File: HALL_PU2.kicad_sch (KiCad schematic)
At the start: 21 parts, among them Q15 AO3400A, Q16 AO3401A, Q17 AO3401A, Q2 AO3400A, Q4 AO3401A, Q5 AO3401A

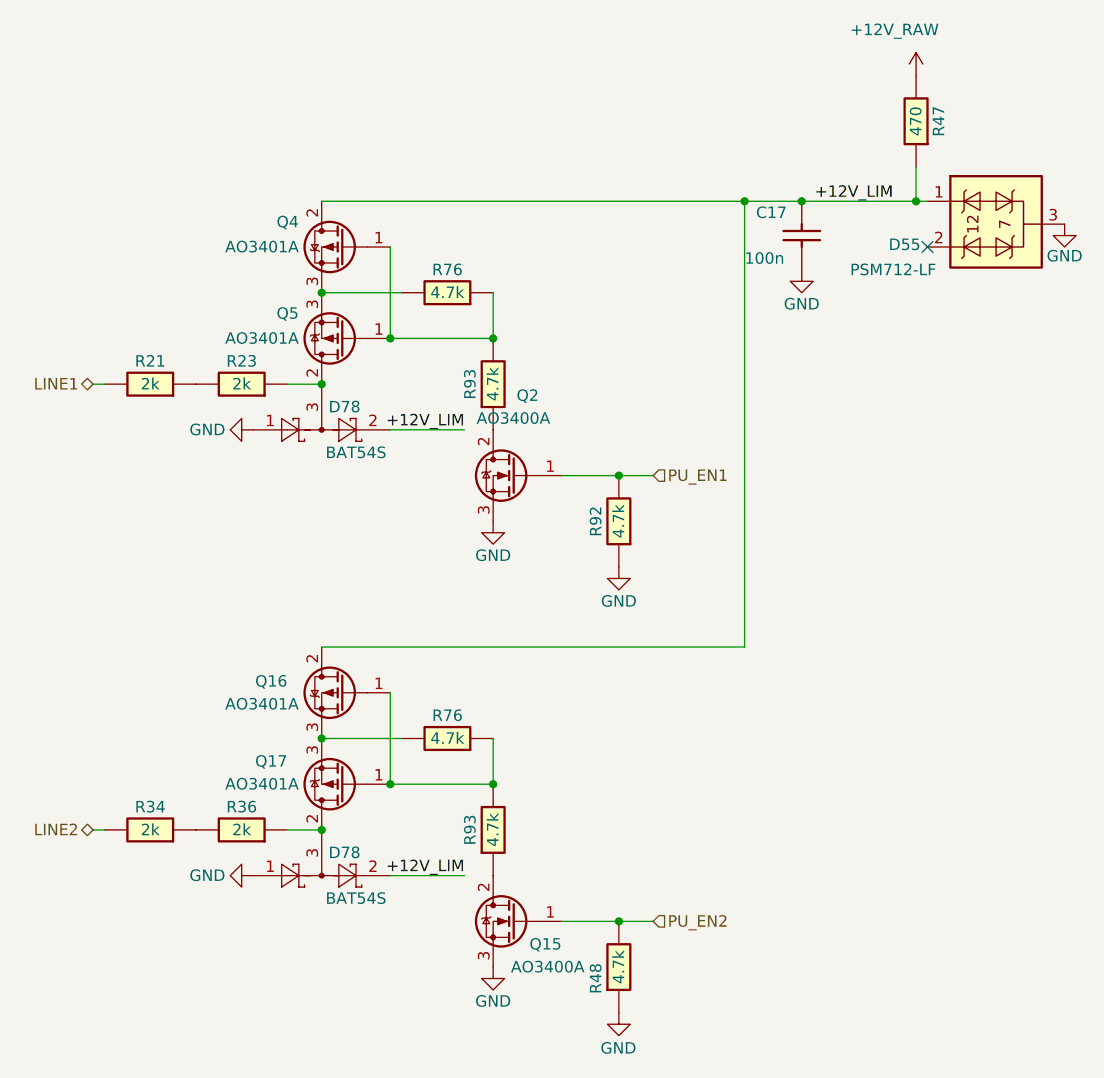
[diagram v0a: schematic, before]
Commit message: Upd PCB
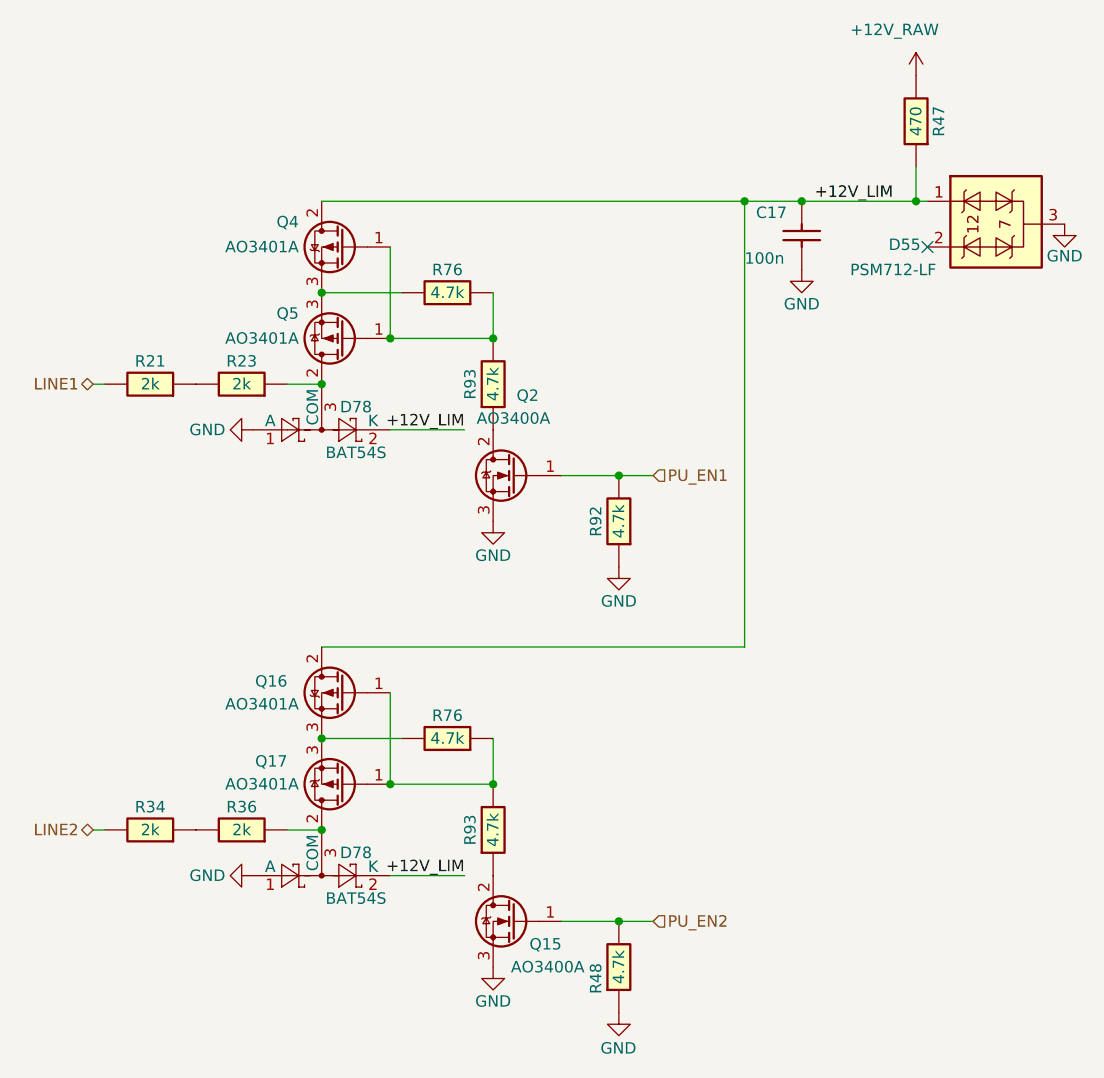
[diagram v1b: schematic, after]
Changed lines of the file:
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@@
         )
         (path "/63d2dd9f-d5ff-4811-a88d-0ba932475460/c3180053-8962-408f-82db-60bcd283a2bd"
-          (reference "R76") (unit 1)
+          (reference "R47") (unit 1)
         )
       )
@@
         )
         (path "/63d2dd9f-d5ff-4811-a88d-0ba932475460/c3180053-8962-408f-82db-60bcd283a2bd"
-          (reference "R93") (unit 1)
+          (reference "R48") (unit 1)
         )
       )
@@
         )
         (path "/63d2dd9f-d5ff-4811-a88d-0ba932475460/c3180053-8962-408f-82db-60bcd283a2bd"
-          (reference "#PWR026") (unit 1)
+          (reference "#PWR038") (unit 1)
         )
       )
@@
         )
         (path "/63d2dd9f-d5ff-4811-a88d-0ba932475460/c3180053-8962-408f-82db-60bcd283a2bd"
-          (reference "Q15") (unit 1)
+          (reference "Q17") (unit 1)
         )
       )
@@
         )
         (path "/63d2dd9f-d5ff-4811-a88d-0ba932475460/c3180053-8962-408f-82db-60bcd283a2bd"
-          (reference "R34") (unit 1)
+          (reference "R23") (unit 1)
         )
       )
@@
         )
         (path "/63d2dd9f-d5ff-4811-a88d-0ba932475460/c3180053-8962-408f-82db-60bcd283a2bd"
-          (reference "#PWR026") (unit 1)
+          (reference "#PWR070") (unit 1)
         )
       )
@@
         )
         (path "/63d2dd9f-d5ff-4811-a88d-0ba932475460/c3180053-8962-408f-82db-60bcd283a2bd"
-          (reference "#PWR070") (unit 1)
+          (reference "#PWR092") (unit 1)
         )
       )
@@
         )
         (path "/63d2dd9f-d5ff-4811-a88d-0ba932475460/c3180053-8962-408f-82db-60bcd283a2bd"
-          (reference "Q2") (unit 1)
+          (reference "Q16") (unit 1)
         )
       )
@@
         )
         (path "/63d2dd9f-d5ff-4811-a88d-0ba932475460/c3180053-8962-408f-82db-60bcd283a2bd"
-          (reference "#PWR0126") (unit 1)
+          (reference "#PWR091") (unit 1)
         )
       )
@@
         )
         (path "/63d2dd9f-d5ff-4811-a88d-0ba932475460/c3180053-8962-408f-82db-60bcd283a2bd"
-          (reference "#PWR0280") (unit 1)
+          (reference "#PWR026") (unit 1)
         )
       )
@@
         )
         (path "/63d2dd9f-d5ff-4811-a88d-0ba932475460/c3180053-8962-408f-82db-60bcd283a2bd"
-          (reference "Q17") (unit 1)
+          (reference "Q15") (unit 1)
         )
       )
@@
         )
         (path "/63d2dd9f-d5ff-4811-a88d-0ba932475460/c3180053-8962-408f-82db-60bcd283a2bd"
-          (reference "R23") (unit 1)
+          (reference "R34") (unit 1)
         )
       )
@@
         )
         (path "/63d2dd9f-d5ff-4811-a88d-0ba932475460/c3180053-8962-408f-82db-60bcd283a2bd"
-          (reference "R92") (unit 1)
+          (reference "R63") (unit 1)
         )
       )
@@
         )
         (path "/63d2dd9f-d5ff-4811-a88d-0ba932475460/c3180053-8962-408f-82db-60bcd283a2bd"
-          (reference "#PWR029") (unit 1)
+          (reference "#PWR039") (unit 1)
         )
       )
@@
         )
         (path "/63d2dd9f-d5ff-4811-a88d-0ba932475460/c3180053-8962-408f-82db-60bcd283a2bd"
-          (reference "R93") (unit 1)
+          (reference "R62") (unit 1)
         )
       )
@@
         )
         (path "/63d2dd9f-d5ff-4811-a88d-0ba932475460/c3180053-8962-408f-82db-60bcd283a2bd"
-          (reference "#PWR038") (unit 1)
+          (reference "#PWR093") (unit 1)
         )
       )
@@
         )
         (path "/63d2dd9f-d5ff-4811-a88d-0ba932475460/c3180053-8962-408f-82db-60bcd283a2bd"
-          (reference "#PWR039") (unit 1)
+          (reference "#PWR095") (unit 1)
         )
       )
@@
         )
         (path "/63d2dd9f-d5ff-4811-a88d-0ba932475460/c3180053-8962-408f-82db-60bcd283a2bd"
-          (reference "R48") (unit 1)
+          (reference "R64") (unit 1)
         )
       )
@@
   (symbol (lib_id "Diode:BAT54S") (at 125.73 64.77 0) (mirror x) (unit 1)
     (in_bom yes) (on_board yes) (dnp no)
-    (property "Reference" "D78" (at 128.27 62.23 0)
+    (property "Reference" "D78" (at 129.54 62.23 0)
       (effects (font (size 1.27 1.27)))
     )
@@
         )
         (path "/63d2dd9f-d5ff-4811-a88d-0ba932475460/c3180053-8962-408f-82db-60bcd283a2bd"
-          (reference "D78") (unit 1)
+          (reference "D28") (unit 1)
         )
       )
@@
         )
         (path "/63d2dd9f-d5ff-4811-a88d-0ba932475460/c3180053-8962-408f-82db-60bcd283a2bd"
-          (reference "Q16") (unit 1)
+          (reference "Q5") (unit 1)
         )
       )
@@
         )
         (path "/63d2dd9f-d5ff-4811-a88d-0ba932475460/c3180053-8962-408f-82db-60bcd283a2bd"
-          (reference "#PWR0280") (unit 1)
+          (reference "#PWR029") (unit 1)
         )
       )
@@
   (symbol (lib_id "Diode:BAT54S") (at 125.73 114.3 0) (mirror x) (unit 1)
     (in_bom yes) (on_board yes) (dnp no)
-    (property "Reference" "D78" (at 128.27 111.76 0)
+    (property "Reference" "D78" (at 129.54 111.76 0)
       (effects (font (size 1.27 1.27)))
     )
@@
         )
         (path "/63d2dd9f-d5ff-4811-a88d-0ba932475460/c3180053-8962-408f-82db-60bcd283a2bd"
-          (reference "D78") (unit 1)
+          (reference "D29") (unit 1)
         )
       )
@@
         )
         (path "/63d2dd9f-d5ff-4811-a88d-0ba932475460/c3180053-8962-408f-82db-60bcd283a2bd"
-          (reference "Q4") (unit 1)
+          (reference "Q2") (unit 1)
         )
       )
@@
         )
         (path "/63d2dd9f-d5ff-4811-a88d-0ba932475460/c3180053-8962-408f-82db-60bcd283a2bd"
-          (reference "D55") (unit 1)
+          (reference "D30") (unit 1)
         )
       )
@@
         )
         (path "/63d2dd9f-d5ff-4811-a88d-0ba932475460/c3180053-8962-408f-82db-60bcd283a2bd"
-          (reference "R47") (unit 1)
+          (reference "R65") (unit 1)
         )
       )
@@
         )
         (path "/63d2dd9f-d5ff-4811-a88d-0ba932475460/c3180053-8962-408f-82db-60bcd283a2bd"
-          (reference "C17") (unit 1)
+          (reference "C6") (unit 1)
         )
       )
@@
         )
         (path "/63d2dd9f-d5ff-4811-a88d-0ba932475460/c3180053-8962-408f-82db-60bcd283a2bd"
-          (reference "R76") (unit 1)
+          (reference "R61") (unit 1)
         )
       )
@@
         )
         (path "/63d2dd9f-d5ff-4811-a88d-0ba932475460/c3180053-8962-408f-82db-60bcd283a2bd"
-          (reference "Q5") (unit 1)
-        )
-      )
+          (reference "Q4") (unit 1)
+        )
+      )

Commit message: Shortage fix
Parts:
- D78: LCSC C408389 -> C47546
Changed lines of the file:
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@@
       (effects (font (size 1.27 1.27)) hide)
     )
-    (property "LCSC" "C408389" (at 125.73 64.77 0)
+    (property "LCSC" "C47546" (at 125.73 64.77 0)
       (effects (font (size 1.27 1.27)) hide)
     )
@@
       (effects (font (size 1.27 1.27)) hide)
     )
-    (property "LCSC" "C408389" (at 125.73 114.3 0)
+    (property "LCSC" "C47546" (at 125.73 114.3 0)
       (effects (font (size 1.27 1.27)) hide)
     )

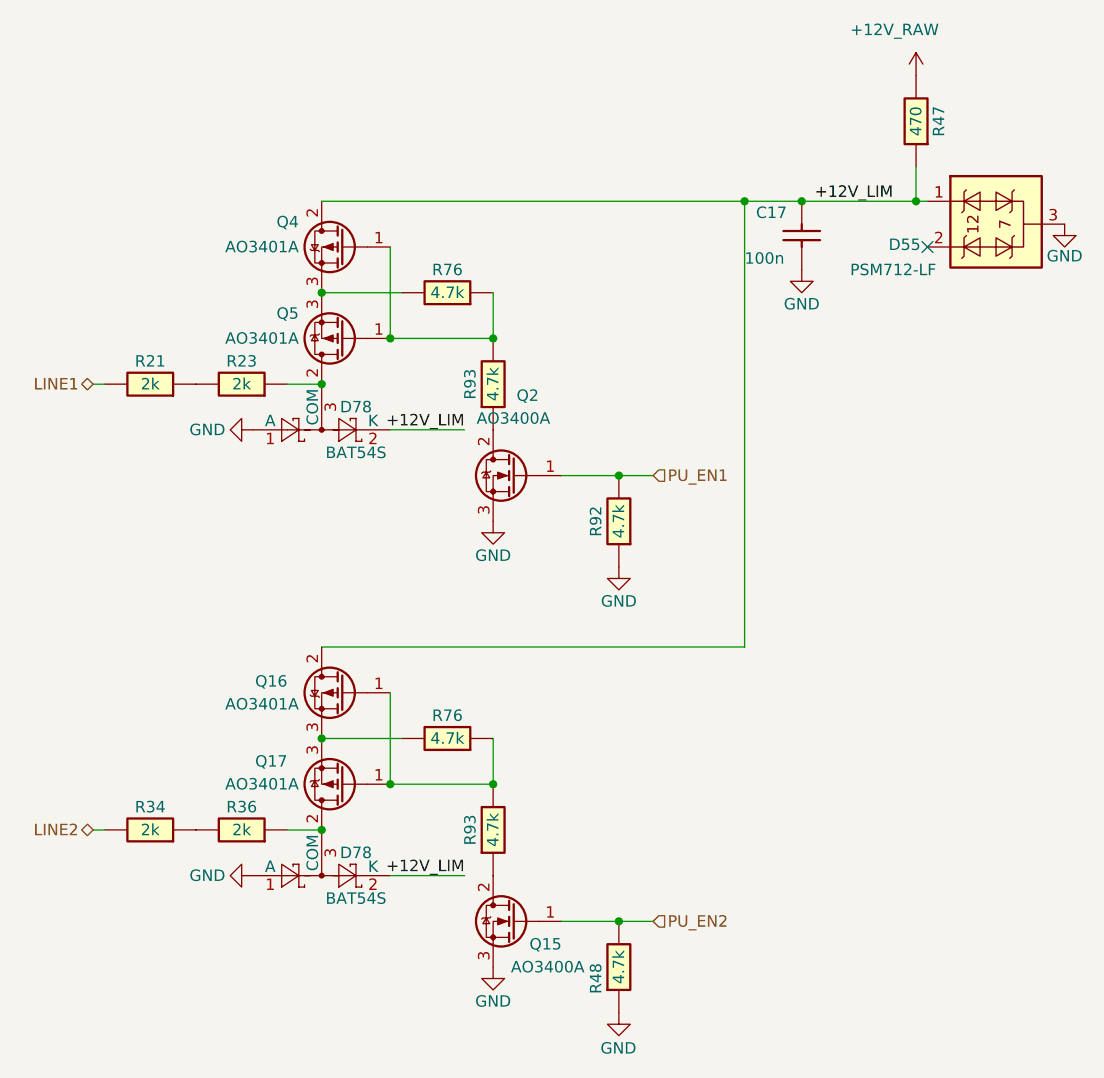
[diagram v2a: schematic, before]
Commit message: Fab preview
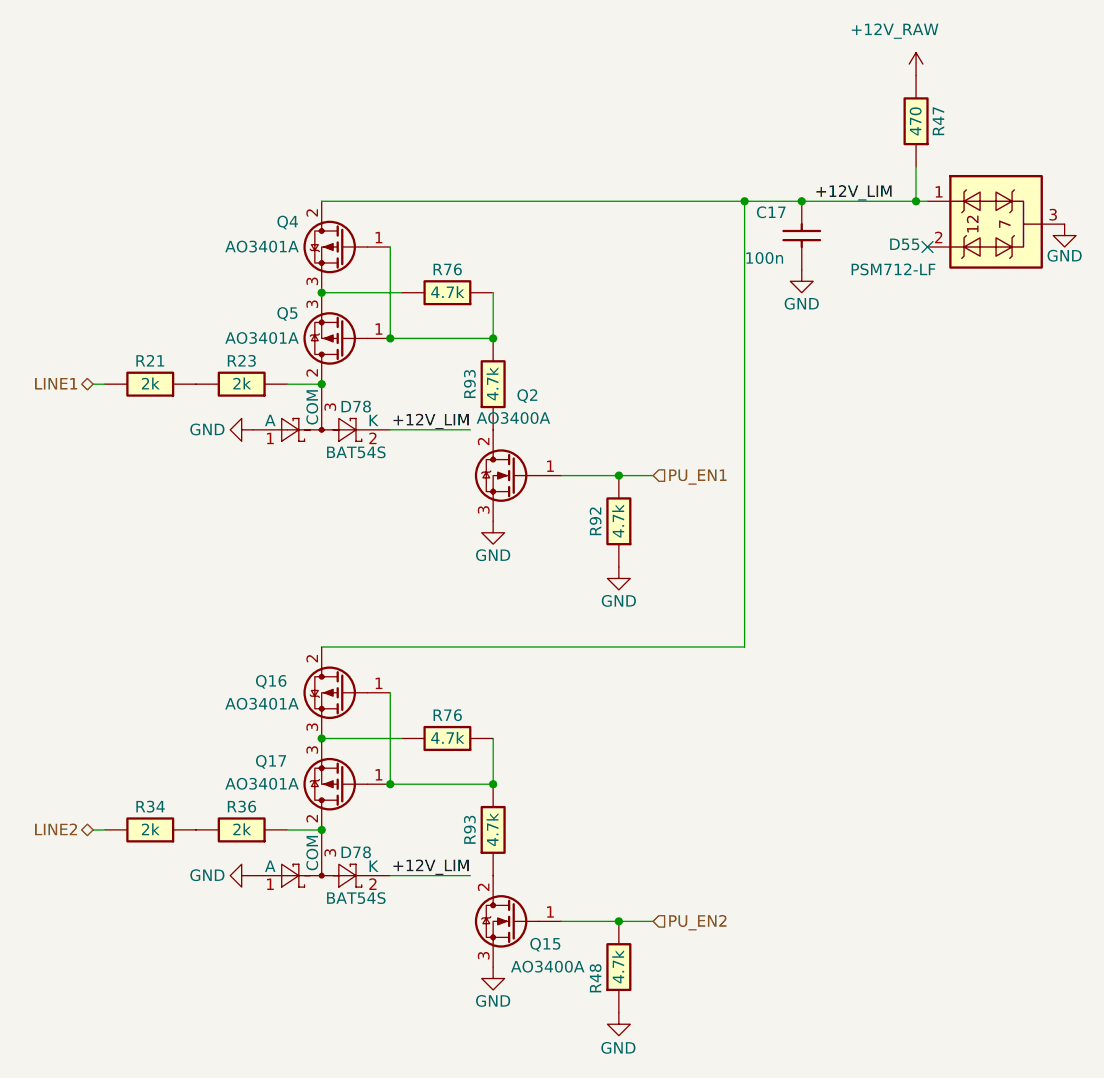
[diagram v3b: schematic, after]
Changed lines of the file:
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@@
     (stroke (width 0) (type default))
   )
-  (wire (pts (xy 141.605 64.77) (xy 133.35 64.77))
+  (wire (pts (xy 142.24 64.77) (xy 133.35 64.77))
     (stroke (width 0) (type default))
   )
@@
   )
   (wire (pts (xy 100.33 59.69) (xy 101.6 59.69))
+    (stroke (width 0) (type default))
+  )
+  (wire (pts (xy 133.35 114.3) (xy 142.24 114.3))
     (stroke (width 0) (type default))
   )
@@
     (stroke (width 0) (type default))
   )
-  (wire (pts (xy 141.605 114.3) (xy 133.35 114.3))
-    (stroke (width 0) (type default))
-  )
   (wire (pts (xy 152.4 119.38) (xy 158.75 119.38))
     (stroke (width 0) (type default))
   )
-  (label "+12V_LIM" (at 141.605 64.77 180) (fields_autoplaced)
+  (label "+12V_LIM" (at 142.24 64.77 180) (fields_autoplaced)
     (effects (font (size 1.27 1.27)) (justify right bottom))
   )
@@
     (effects (font (size 1.27 1.27)) (justify right bottom))
   )
-  (label "+12V_LIM" (at 141.605 114.3 180) (fields_autoplaced)
+  (label "+12V_LIM" (at 142.24 114.3 180) (fields_autoplaced)
     (effects (font (size 1.27 1.27)) (justify right bottom))
   )
